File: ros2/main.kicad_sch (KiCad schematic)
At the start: 54 parts, among them J1 Battery Conn_01x02, J2 BMS_input, J3 BMS_output, J4 Conn_01x03, J5 SW_CONNECTOR, J6 ACS_IN, J7 ACS_POWER_OUT, SW1 MRS-101, U1 ESP32-DEVKIT-V1, U2 TB6612NFG, U3 TB6612NFG, U4 TB6612NFG, U5 TB6612NFG, U6 TXS0108E, U7 ACS712_MODULE, U8 XL63070

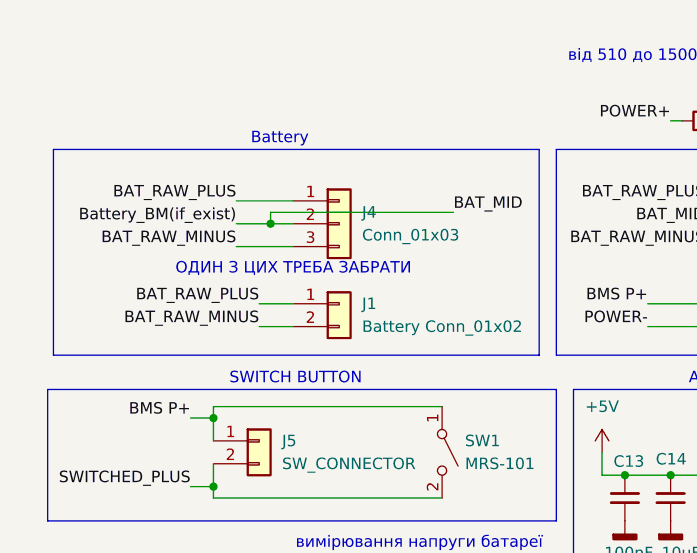
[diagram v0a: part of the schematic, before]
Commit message: saved details
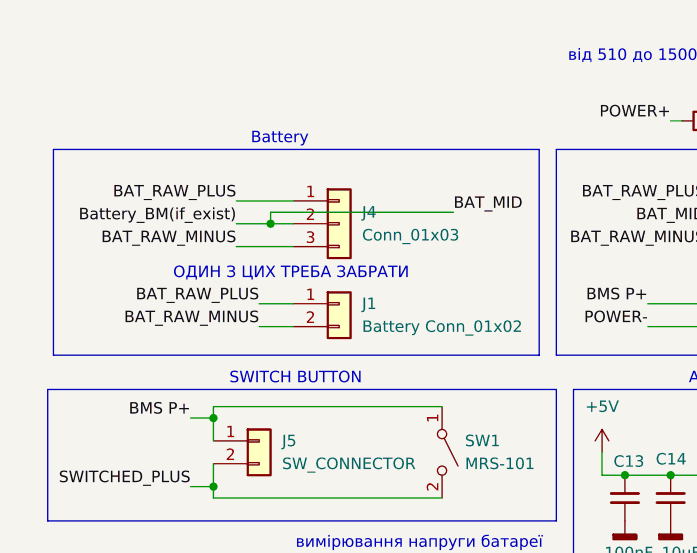
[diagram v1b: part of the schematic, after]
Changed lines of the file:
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@@
 	(text "ОДИН З ЦИХ ТРЕБА ЗАБРАТИ"
 		(exclude_from_sim no)
-		(at 40.64 38.1 0)
+		(at 40.386 38.608 0)
 		(effects
 			(font

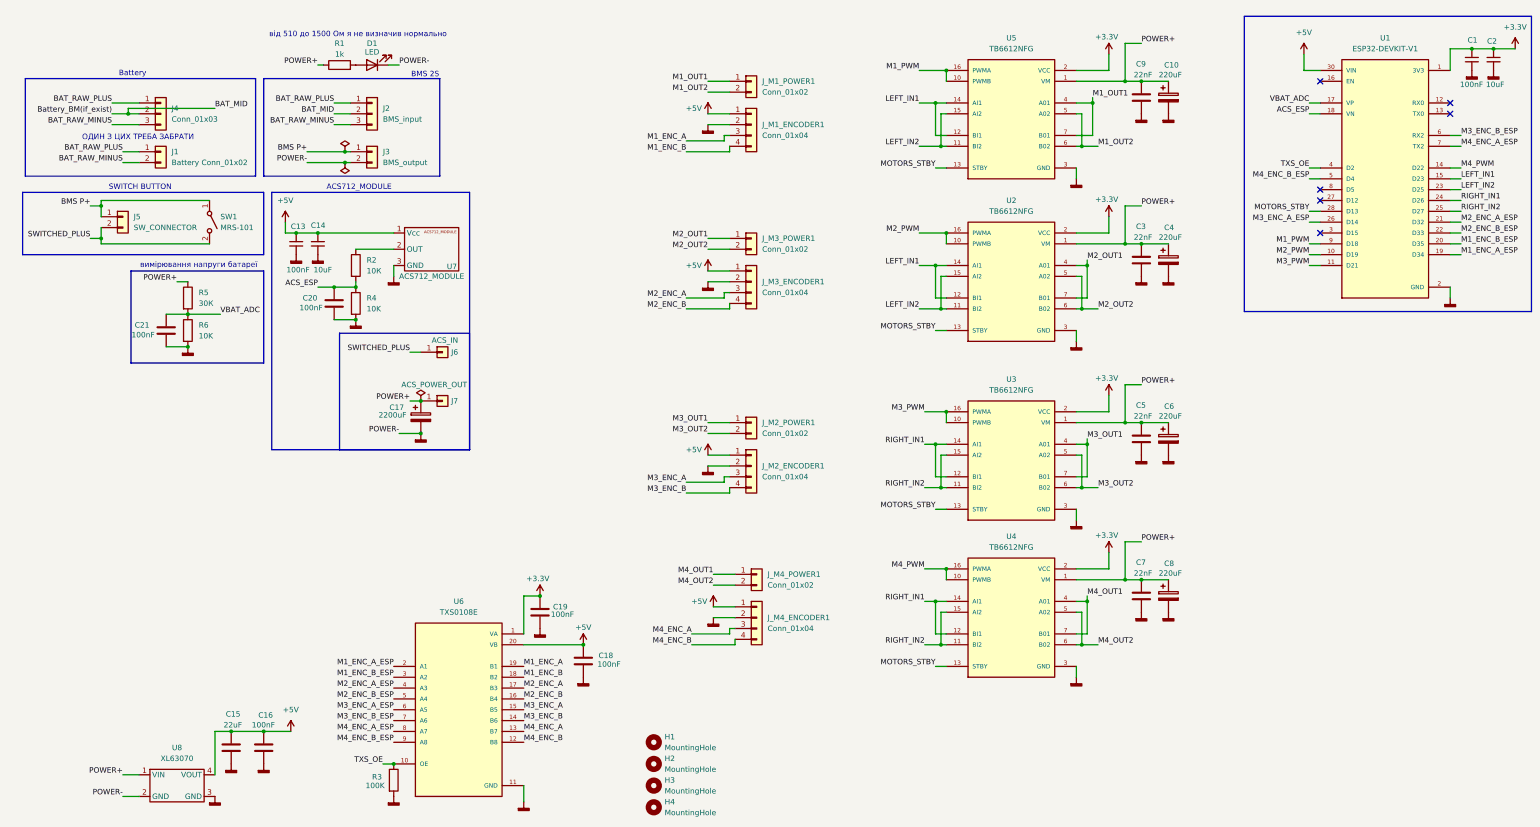
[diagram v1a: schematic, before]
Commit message: prettier fix
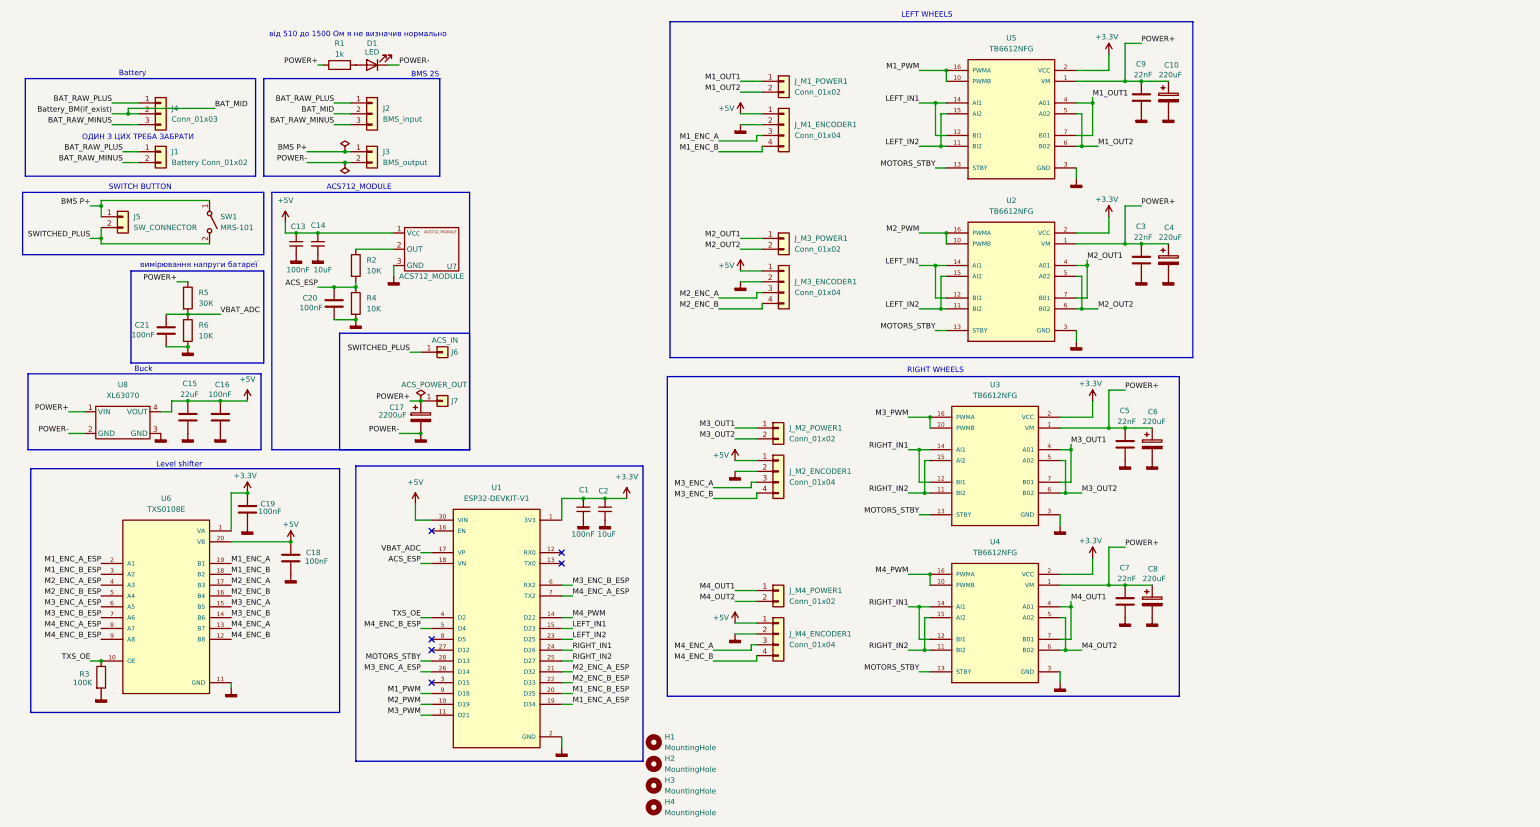
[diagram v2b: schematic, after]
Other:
- note added: "Buck"
- note added: "LEFT WHEELS"
- note added: "Level shifter"
- note added: "RIGHT WHEELS"
- moved on the sheet: C1, C15, C16, C18, C19, C2, C5, C6, C7, C8, J_M1_ENCODER1, J_M1_POWER1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
